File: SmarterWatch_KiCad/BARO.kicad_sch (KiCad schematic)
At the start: 1 part

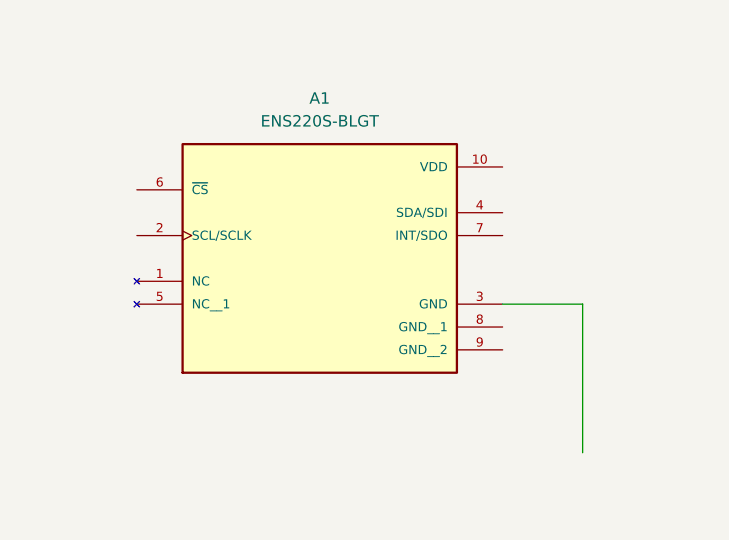
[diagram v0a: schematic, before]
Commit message: baro progress
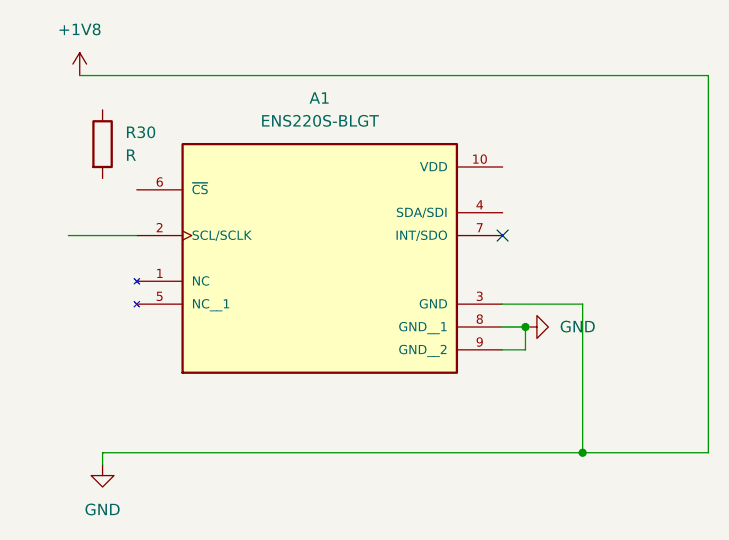
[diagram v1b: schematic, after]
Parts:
- added R30: R, symbol Device:R
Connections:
- net +1V8: now reaches A1.3 (GND)
- net +1V8: now also A1.8 (GND__1), A1.9 (GND__2)
- no-connect marks 0 -> 1

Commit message: Magnetometor sheet
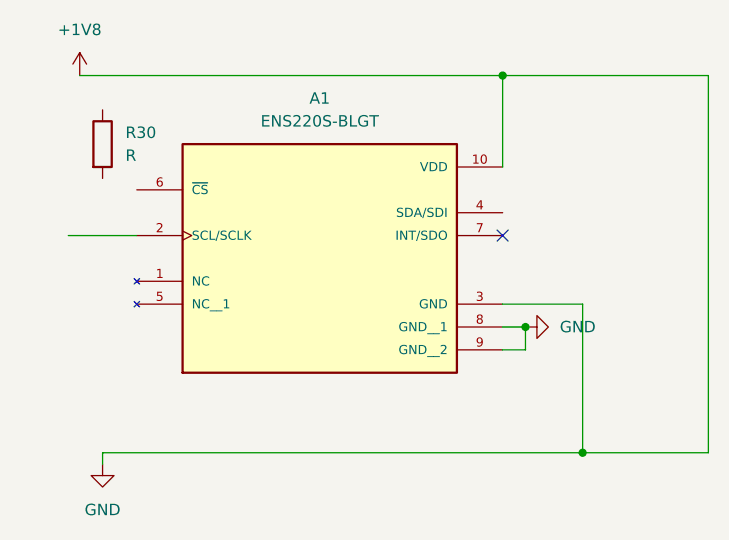
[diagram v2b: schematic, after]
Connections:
- net +1V8: now also A1.10 (VDD)
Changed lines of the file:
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@@
+		(color 0 0 0 0)
+	)
+	(junction
+		(at 158.75 90.17)
+		(diameter 0)
 		(color 0 0 0 0)
 	)
@@
 	(wire
 		(pts
-			(xy 111.76 90.17) (xy 181.61 90.17)
+			(xy 111.76 90.17) (xy 158.75 90.17)
 		)
 		(stroke
@@
 	(wire
 		(pts
+			(xy 158.75 90.17) (xy 181.61 90.17)
+		)
+		(stroke
+			(width 0)
+			(type default)
+		)
+	)
+	(wire
+		(pts
 			(xy 114.3 132.08) (xy 167.64 132.08)
 		)
 		(stroke
+			(width 0)
+			(type default)
+		)
+	)
+	(wire
+		(pts
+			(xy 158.75 90.17) (xy 158.75 100.33)
+		)
+		(stroke

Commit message: Baro
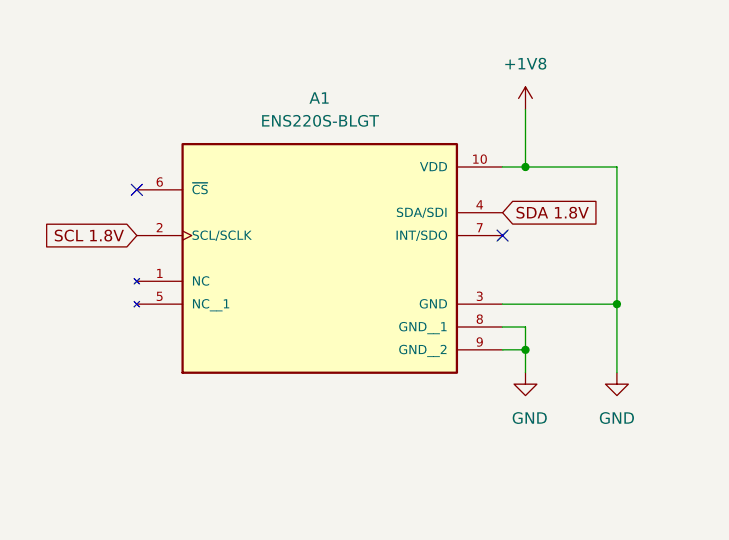
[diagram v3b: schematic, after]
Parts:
- removed R30: R, symbol Device:R
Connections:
- net SCL 1.8V: now reaches A1.2 (SCL/SCLK)
- net SDA 1.8V: now reaches A1.4 (SDA/SDI)
- no-connect marks 1 -> 2
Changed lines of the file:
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@@
 	(paper "A4")
 	(junction
-		(at 161.29 118.11)
+		(at 171.45 115.57)
 		(diameter 0)
 		(color 0 0 0 0)
 	)
 	(junction
-		(at 167.64 132.08)
+		(at 161.29 120.65)
 		(diameter 0)
 		(color 0 0 0 0)
 	)
 	(junction
-		(at 158.75 90.17)
+		(at 161.29 100.33)
 		(diameter 0)
 		(color 0 0 0 0)
 	)
 	(no_connect
+		(at 118.11 102.87)
+	)
+	(no_connect
 		(at 158.75 107.95)
 	)
 	(wire
 		(pts
+			(xy 161.29 123.19) (xy 161.29 120.65)
+		)
+		(stroke
+			(width 0)
+			(type default)
+		)
+	)
+	(wire
+		(pts
 			(xy 158.75 120.65) (xy 161.29 120.65)
 		)
@@
 	(wire
 		(pts
-			(xy 158.75 115.57) (xy 167.64 115.57)
+			(xy 158.75 115.57) (xy 171.45 115.57)
 		)
 		(stroke
@@
 	(wire
 		(pts
-			(xy 111.76 90.17) (xy 158.75 90.17)
-		)
-		(stroke
-			(width 0)
-			(type default)
-		)
-	)
-	(wire
-		(pts
-			(xy 110.49 107.95) (xy 118.11 107.95)
-		)
-		(stroke
-			(width 0)
-			(type default)
-		)
-	)
-	(wire
-		(pts
-			(xy 114.3 132.08) (xy 114.3 133.35)
-		)
-		(stroke
-			(width 0)
-			(type default)
-		)
-	)
-	(wire
-		(pts
-			(xy 167.64 132.08) (xy 181.61 132.08)
+			(xy 161.29 100.33) (xy 158.75 100.33)
 		)
 		(stroke
@@
 	(wire
 		(pts
-			(xy 158.75 90.17) (xy 181.61 90.17)
-		)
-		(stroke
-			(width 0)
-			(type default)
-		)
-	)
-	(wire
-		(pts
-			(xy 114.3 132.08) (xy 167.64 132.08)
-		)
-		(stroke
-			(width 0)
-			(type default)
-		)
-	)
-	(wire
-		(pts
-			(xy 158.75 90.17) (xy 158.75 100.33)
-		)
-		(stroke
-			(width 0)
-			(type default)
-		)
-	)
-	(wire
-		(pts
-			(xy 181.61 132.08) (xy 181.61 90.17)
-		)
-		(stroke
-			(width 0)
-			(type default)
-		)
-	)
-	(wire
-		(pts
-			(xy 167.64 115.57) (xy 167.64 132.08)
-		)
-		(stroke
-			(width 0)
-			(type default)
+			(xy 161.29 100.33) (xy 171.45 100.33)
+		)
+		(stroke
+			(width 0)
+			(type default)
+		)
+	)
+	(wire
+		(pts
+			(xy 161.29 93.98) (xy 161.29 100.33)
+		)
+		(stroke
+			(width 0)
+			(type default)
+		)
+	)
+	(wire
+		(pts
+			(xy 171.45 115.57) (xy 171.45 100.33)
+		)
+		(stroke
+			(width 0)
+			(type default)
+		)
+	)
+	(wire
+		(pts
+			(xy 171.45 115.57) (xy 171.45 123.19)
+		)
+		(stroke
+			(width 0)
+			(type default)
+		)
+	)
+	(global_label "SDA 1.8V"
+		(shape input)
+		(at 158.75 105.41 0)
+		(fields_autoplaced yes)
+		(effects
+			(font
+				(size 1.27 1.27)
+			)
+			(justify left)
+		)
+		(property "Intersheetrefs" "${INTERSHEET_REFS}"
+			(at 170.3833 105.41 0)
+			(effects
+				(font
+					(size 1.27 1.27)
+				)
+				(justify left)
+				(hide yes)
+			)
+		)
+	)
+	(global_label "SCL 1.8V"
+		(shape input)
+		(at 118.11 107.95 180)
+		(fields_autoplaced yes)
+		(effects
+			(font
+				(size 1.27 1.27)
+			)
+			(justify right)
+		)
+		(property "Intersheetrefs" "${INTERSHEET_REFS}"
+			(at 106.5372 107.95 0)
+			(effects
+				(font
+					(size 1.27 1.27)
+				)
+				(justify right)
+				(hide yes)
+			)
 		)
 	)
 	(symbol
-		(lib_id "Device:R")
-		(at 114.3 97.79 0)
+		(lib_id "power:GND")
+		(at 161.29 123.19 0)
 		(unit 1)
 		(exclude_from_sim no)
@@
 		(on_board yes)
 		(dnp no)
-		(fields_autoplaced yes)
-		(property "Reference" "R30"
-			(at 116.84 96.5199 0)
+		(property "Reference" "#PWR077"
+			(at 161.29 129.54 0)
+			(effects
+				(font
+					(size 1.27 1.27)
+				)
+				(hide yes)
+			)
+		)
+		(property "Value" "GND"
+			(at 159.766 128.27 0)
 			(effects
 				(font
@@
 			)
 		)
-		(property "Value" "R"
-			(at 116.84 99.0599 0)
-			(effects
-				(font
-					(size 1.27 1.27)
-				)
-				(justify left)
-			)
-		)
 		(property "Footprint" ""
-			(at 112.522 97.79 90)
-			(effects
-				(font
-					(size 1.27 1.27)
-				)
-				(hide yes)
-			)
-		)
-		(property "Datasheet" "~"
-			(at 114.3 97.79 0)
-			(effects
-				(font
-					(size 1.27 1.27)
-				)
-				(hide yes)
-			)
-		)
-		(property "Description" "Resistor"
-			(at 114.3 97.79 0)
-			(effects
-				(font
-					(size 1.27 1.27)
-				)
-				(hide yes)
-			)
-		)
-		(pin "2"
-		)
-		(pin "1"
-		)
-		(instances
-			(project ""
-				(path "/52181fb0-1be8-41da-83b2-7d5a62778ff4/64b56c59-94b5-4fcd-a1b7-d29a8b43cdbf"
-					(reference "R30")
-					(unit 1)
-				)
-			)
-		)
-	)
-	(symbol
-		(lib_id "power:GND")
-		(at 161.29 118.11 90)
-		(unit 1)
-		(exclude_from_sim no)
-		(in_bom yes)
-		(on_board yes)
-		(dnp no)
-		(fields_autoplaced yes)
-		(property "Reference" "#PWR077"
-			(at 167.64 118.11 0)
-			(effects
-				(font
-					(size 1.27 1.27)
-				)
-				(hide yes)
-			)
-		)
-		(property "Value" "GND"
-			(at 165.1 118.1099 90)
-			(effects
-				(font
-					(size 1.27 1.27)
-				)
-				(justify right)
-			)
-		)
-		(property "Footprint" ""
-			(at 161.29 118.11 0)
+			(at 161.29 123.19 0)
 			(effects
 				(font
@@
 		)
 		(property "Datasheet" ""
-			(at 161.29 118.11 0)
+			(at 161.29 123.19 0)
 			(effects
 				(font
@@
 		)
 		(property "Description" "Power symbol creates a global label with name \"GND\" , ground"
-			(at 161.29 118.11 0)
+			(at 161.29 123.19 0)
 			(effects
 				(font
@@
 	(symbol
 		(lib_id "power:+1V8")
-		(at 111.76 90.17 0)
+		(at 161.29 93.98 0)
 		(unit 1)
 		(exclude_from_sim no)
@@
 		(on_board yes)
 		(dnp no)
-		(fields_autoplaced yes)
 		(property "Reference" "#PWR079"
-			(at 111.76 93.98 0)
+			(at 161.29 97.79 0)
 			(effects
 				(font
@@
 		)
 		(property "Value" "+1V8"
-			(at 111.76 85.09 0)
+			(at 161.29 88.9 0)
 			(effects
 				(font
@@
 		)
 		(property "Footprint" ""
-			(at 111.76 90.17 0)
+			(at 161.29 93.98 0)
 			(effects
 				(font
@@
 		)
 		(property "Datasheet" ""
-			(at 111.76 90.17 0)
+			(at 161.29 93.98 0)
 			(effects
 				(font
@@
 		)
 		(property "Description" "Power symbol creates a global label with name \"+1V8\""
-			(at 111.76 90.17 0)
+			(at 161.29 93.98 0)
 			(effects
 				(font
@@
 	(symbol
 		(lib_id "power:GND")
-		(at 114.3 133.35 0)
+		(at 171.45 123.19 0)
 		(unit 1)
 		(exclude_from_sim no)
@@
 		(fields_autoplaced yes)
 		(property "Reference" "#PWR078"
-			(at 114.3 139.7 0)
+			(at 171.45 129.54 0)
 			(effects
 				(font
@@
 		)
 		(property "Value" "GND"
-			(at 114.3 138.43 0)
+			(at 171.45 128.27 0)
 			(effects
 				(font
@@
 		)
 		(property "Footprint" ""
-			(at 114.3 133.35 0)
+			(at 171.45 123.19 0)
 			(effects
 				(font
@@
 		)
 		(property "Datasheet" ""
-			(at 114.3 133.35 0)
+			(at 171.45 123.19 0)
 			(effects
 				(font
@@
 		)
 		(property "Description" "Power symbol creates a global label with name \"GND\" , ground"
-			(at 114.3 133.35 0)
-			(effects
-				(font
+			(at 171.45 123.19 0)
+			(effects
+				(font

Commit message: order
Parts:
- A1: footprint ENS220S-BLGT:XDCR_ENS220S-BLGT -> Package_LGA:ST_HLGA-10_2x2mm_P0.5mm_LayoutBorder3x2y
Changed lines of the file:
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@@
 			)
 		)
-		(property "Footprint" "ENS220S-BLGT:XDCR_ENS220S-BLGT"
+		(property "Footprint" "Package_LGA:ST_HLGA-10_2x2mm_P0.5mm_LayoutBorder3x2y"
 			(at 138.43 107.95 0)
 			(effects

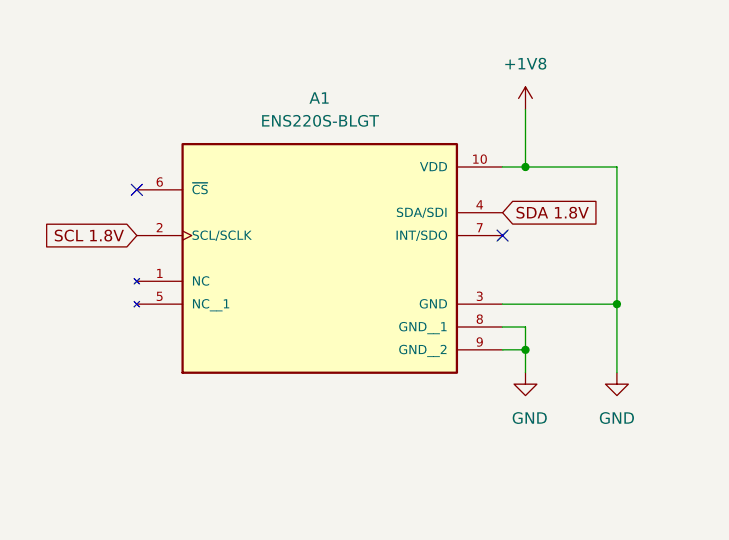
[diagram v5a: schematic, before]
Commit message: foot print stuff
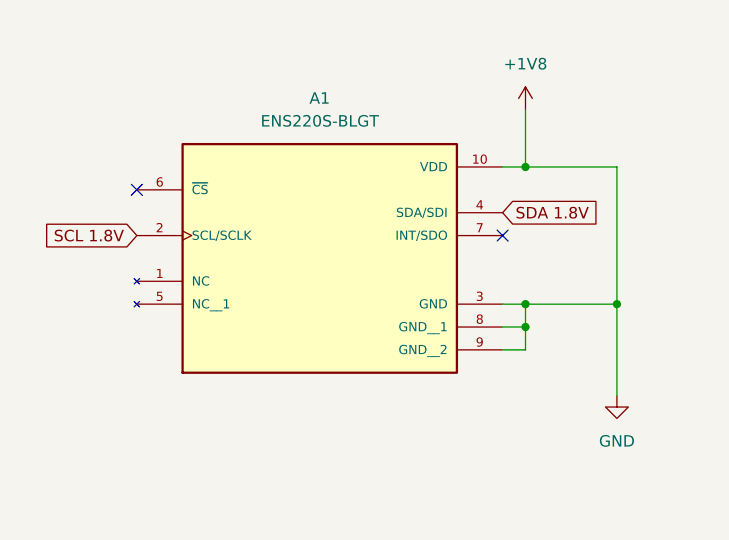
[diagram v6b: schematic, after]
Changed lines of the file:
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@@
 	)
 	(junction
-		(at 161.29 120.65)
+		(at 161.29 115.57)
 		(diameter 0)
 		(color 0 0 0 0)
@@
 		(color 0 0 0 0)
 	)
+	(junction
+		(at 161.29 118.11)
+		(diameter 0)
+		(color 0 0 0 0)
+	)
 	(no_connect
 		(at 118.11 102.87)
@@
 	(wire
 		(pts
-			(xy 161.29 123.19) (xy 161.29 120.65)
+			(xy 161.29 115.57) (xy 171.45 115.57)
 		)
 		(stroke
@@
 	(wire
 		(pts
-			(xy 158.75 115.57) (xy 171.45 115.57)
+			(xy 158.75 115.57) (xy 161.29 115.57)
 		)
 		(stroke
@@
 	(wire
 		(pts
+			(xy 161.29 115.57) (xy 161.29 118.11)
+		)
+		(stroke
+			(width 0)
+			(type default)
+		)
+	)
+	(wire
+		(pts
 			(xy 161.29 100.33) (xy 171.45 100.33)
 		)
@@
 	(wire
 		(pts
-			(xy 171.45 115.57) (xy 171.45 123.19)
+			(xy 171.45 115.57) (xy 171.45 125.73)
 		)
 		(stroke
@@
 				(justify right)
 				(hide yes)
-			)
-		)
-	)
-	(symbol
-		(lib_id "power:GND")
-		(at 161.29 123.19 0)
-		(unit 1)
-		(exclude_from_sim no)
-		(in_bom yes)
-		(on_board yes)
-		(dnp no)
-		(property "Reference" "#PWR082"
-			(at 161.29 129.54 0)
-			(effects
-				(font
-					(size 1.27 1.27)
-				)
-				(hide yes)
-			)
-		)
-		(property "Value" "GND"
-			(at 159.766 128.27 0)
-			(effects
-				(font
-					(size 1.27 1.27)
-				)
-				(justify left)
-			)
-		)
-		(property "Footprint" ""
-			(at 161.29 123.19 0)
-			(effects
-				(font
-					(size 1.27 1.27)
-				)
-				(hide yes)
-			)
-		)
-		(property "Datasheet" ""
-			(at 161.29 123.19 0)
-			(effects
-				(font
-					(size 1.27 1.27)
-				)
-				(hide yes)
-			)
-		)
-		(property "Description" "Power symbol creates a global label with name \"GND\" , ground"
-			(at 161.29 123.19 0)
-			(effects
-				(font
-					(size 1.27 1.27)
-				)
-				(hide yes)
-			)
-		)
-		(pin "1"
-		)
-		(instances
-			(project ""
-				(path "/52181fb0-1be8-41da-83b2-7d5a62778ff4/64b56c59-94b5-4fcd-a1b7-d29a8b43cdbf"
-					(reference "#PWR082")
-					(unit 1)
-				)
 			)
 		)
@@
 	(symbol
 		(lib_id "power:GND")
-		(at 171.45 123.19 0)
+		(at 171.45 125.73 0)
 		(unit 1)
 		(exclude_from_sim no)
@@
 		(fields_autoplaced yes)
 		(property "Reference" "#PWR083"
-			(at 171.45 129.54 0)
+			(at 171.45 132.08 0)
 			(effects
 				(font
@@
 		)
 		(property "Value" "GND"
-			(at 171.45 128.27 0)
+			(at 171.45 130.81 0)
 			(effects
 				(font
@@
 		)
 		(property "Footprint" ""
-			(at 171.45 123.19 0)
+			(at 171.45 125.73 0)
 			(effects
 				(font
@@
 		)
 		(property "Datasheet" ""
-			(at 171.45 123.19 0)
+			(at 171.45 125.73 0)
 			(effects
 				(font
@@
 		)
 		(property "Description" "Power symbol creates a global label with name \"GND\" , ground"
-			(at 171.45 123.19 0)
-			(effects
-				(font
+			(at 171.45 125.73 0)
+			(effects
+				(font

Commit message: commiting ts
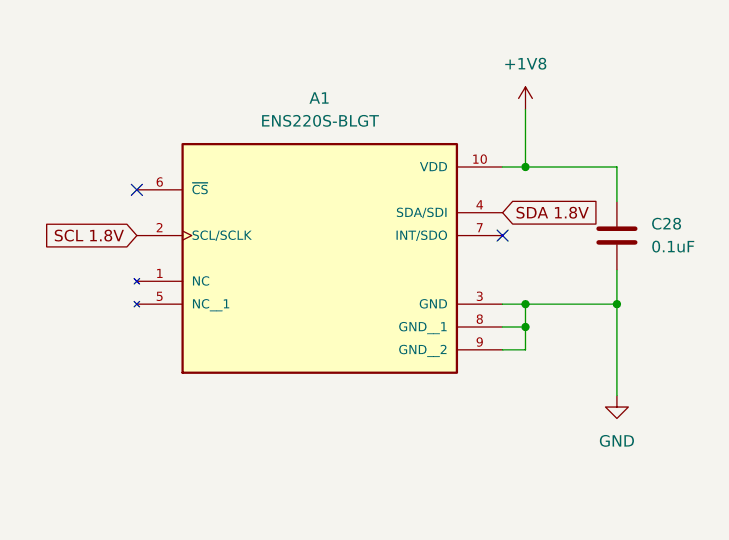
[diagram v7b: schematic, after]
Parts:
- added C28: 0.1uF, Capacitor_SMD:C_0402_1005Metric, symbol Device:C
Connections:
- net +1V8: now also C28.1; no longer A1.3 (GND), A1.8 (GND__1), A1.9 (GND__2)
- new net GND: A1.3 (GND), A1.8 (GND__1), A1.9 (GND__2), C28.2
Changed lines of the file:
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@@
+	(wire
+		(pts
+			(xy 171.45 104.14) (xy 171.45 100.33)
+		)
+		(stroke
+			(width 0)
+			(type default)
+		)
+	)
 	(wire
 		(pts
@@
 	(wire
 		(pts
-			(xy 171.45 115.57) (xy 171.45 100.33)
+			(xy 171.45 115.57) (xy 171.45 111.76)
 		)
 		(stroke
@@
 					(unit 1)
 				)
+			)
+		)
+	)
+	(symbol
+		(lib_id "Device:C")
+		(at 171.45 107.95 0)
+		(unit 1)
+		(exclude_from_sim no)
+		(in_bom yes)
+		(on_board yes)
+		(dnp no)
+		(fields_autoplaced yes)
+		(property "Reference" "C28"
+			(at 175.26 106.6799 0)
+			(effects
+				(font
+					(size 1.27 1.27)
+				)
+				(justify left)
+			)
+		)
+		(property "Value" "0.1uF"
+			(at 175.26 109.2199 0)
+			(effects
+				(font
+					(size 1.27 1.27)
+				)
+				(justify left)
+			)
+		)
+		(property "Footprint" "Capacitor_SMD:C_0402_1005Metric"
+			(at 172.4152 111.76 0)
+			(effects
+				(font
+					(size 1.27 1.27)
+				)
+				(hide yes)
+			)
+		)
+		(property "Datasheet" "~"
+			(at 171.45 107.95 0)
+			(effects
+				(font
+					(size 1.27 1.27)
+				)
+				(hide yes)
+			)
+		)
+		(property "Description" "Unpolarized capacitor"
+			(at 171.45 107.95 0)
+			(effects
+				(font
+					(size 1.27 1.27)
+				)
+				(hide yes)
+			)
+		)
+		(pin "1"
+		)
+		(pin "2"
+		)
+		(instances
+			(project ""
+				(path "/52181fb0-1be8-41da-83b2-7d5a62778ff4/64b56c59-94b5-4fcd-a1b7-d29a8b43cdbf"
+					(reference "C28")
+					(unit 1)
+				)

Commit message: update
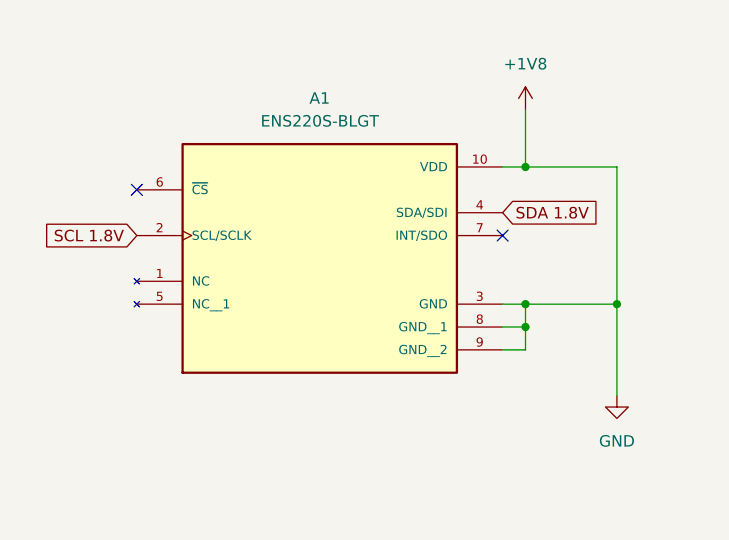
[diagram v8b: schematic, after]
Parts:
- removed C28: 0.1uF, Capacitor_SMD:C_0402_1005Metric, symbol Device:C
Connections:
- net GND is gone; now on net +1V8: A1.3 (GND), A1.8 (GND__1), A1.9 (GND__2)
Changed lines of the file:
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@@
-	(wire
-		(pts
-			(xy 171.45 104.14) (xy 171.45 100.33)
-		)
-		(stroke
-			(width 0)
-			(type default)
-		)
-	)
 	(wire
 		(pts
@@
 	(wire
 		(pts
-			(xy 171.45 115.57) (xy 171.45 111.76)
+			(xy 171.45 115.57) (xy 171.45 100.33)
 		)
 		(stroke
@@
 					(unit 1)
 				)
-			)
-		)
-	)
-	(symbol
-		(lib_id "Device:C")
-		(at 171.45 107.95 0)
-		(unit 1)
-		(exclude_from_sim no)
-		(in_bom yes)
-		(on_board yes)
-		(dnp no)
-		(fields_autoplaced yes)
-		(property "Reference" "C28"
-			(at 175.26 106.6799 0)
-			(effects
-				(font
-					(size 1.27 1.27)
-				)
-				(justify left)
-			)
-		)
-		(property "Value" "0.1uF"
-			(at 175.26 109.2199 0)
-			(effects
-				(font
-					(size 1.27 1.27)
-				)
-				(justify left)
-			)
-		)
-		(property "Footprint" "Capacitor_SMD:C_0402_1005Metric"
-			(at 172.4152 111.76 0)
-			(effects
-				(font
-					(size 1.27 1.27)
-				)
-				(hide yes)
-			)
-		)
-		(property "Datasheet" "~"
-			(at 171.45 107.95 0)
-			(effects
-				(font
-					(size 1.27 1.27)
-				)
-				(hide yes)
-			)
-		)
-		(property "Description" "Unpolarized capacitor"
-			(at 171.45 107.95 0)
-			(effects
-				(font
-					(size 1.27 1.27)
-				)
-				(hide yes)
-			)
-		)
-		(pin "1"
-		)
-		(pin "2"
-		)
-		(instances
-			(project ""
-				(path "/52181fb0-1be8-41da-83b2-7d5a62778ff4/64b56c59-94b5-4fcd-a1b7-d29a8b43cdbf"
-					(reference "C28")
-					(unit 1)
-				)
